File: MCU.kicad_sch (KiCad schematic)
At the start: 34 parts, among them J1 USB_C_Receptacle_USB2.0_16P, SW1 SW_Push, SW2 SW_Push, U1 RP2040, U2 W25Q128JVS, Y1 Crystal_GND24

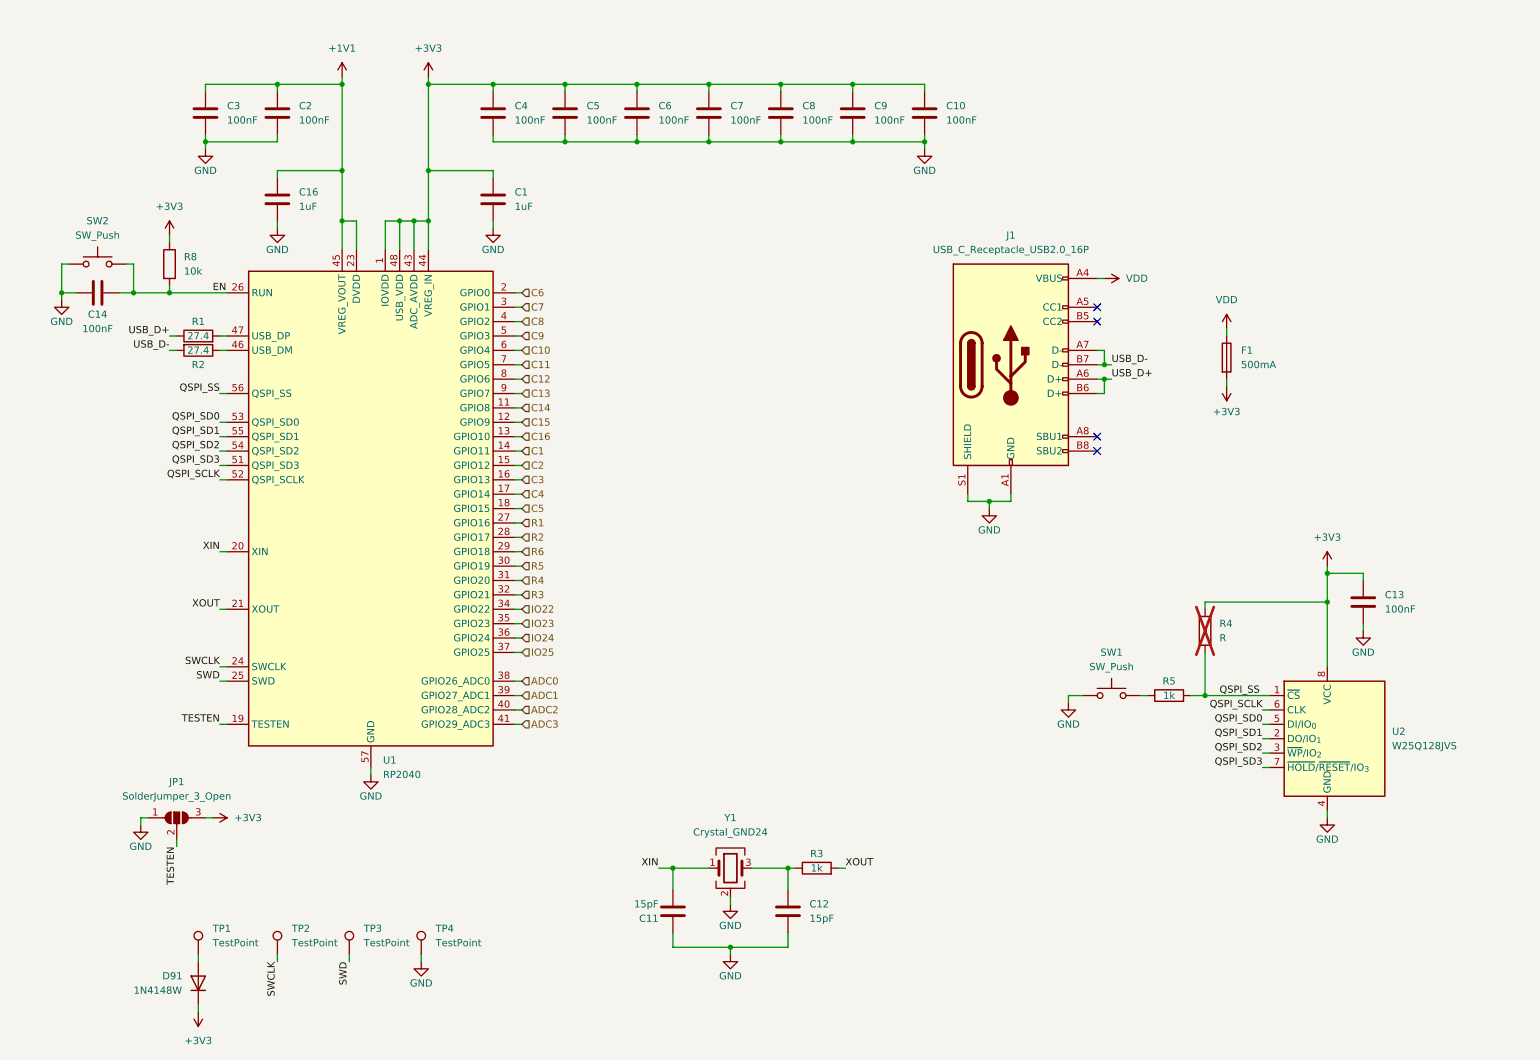
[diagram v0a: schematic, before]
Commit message: Finished V0.1
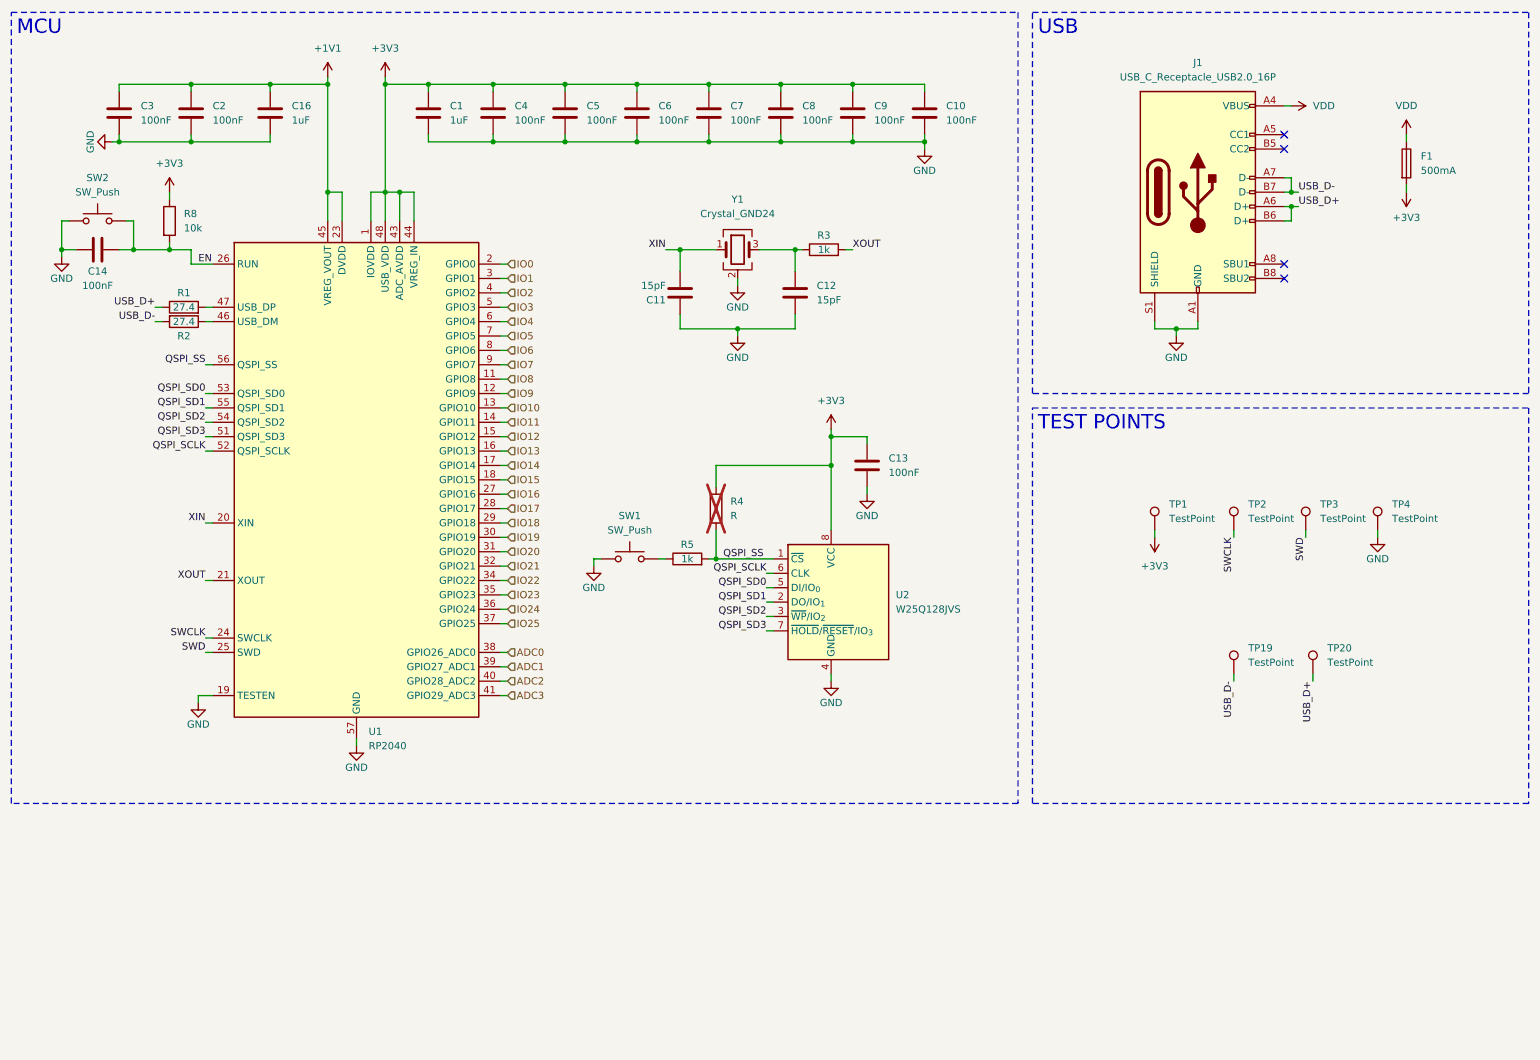
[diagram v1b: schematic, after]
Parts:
- removed D91: 1N4148W, Diode_SMD:D_SOD-123, symbol Diode:1N4148W
- removed JP1: SolderJumper_3_Open, Jumper:SolderJumper-3_P1.3mm_Open_Pad1.0x1.5mm, symbol Jumper:SolderJumper_3_Open
- added TP19, TP20: TestPoint, TestPoint:TestPoint_Pad_D1.0mm, symbol Connector:TestPoint
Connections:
- net TESTEN is gone; now on net GND: U1.19 (TESTEN)
- net +3V3: now also TP1.1
- net USB_D+: now also TP20.1
- net USB_D-: now also TP19.1
- net C1 renamed IO11
- net C10 renamed IO4
- net C11 renamed IO5
- net C12 renamed IO6
- net C13 renamed IO7
- net C14 renamed IO8
- net C15 renamed IO9
- net C16 renamed IO10
- net C2 renamed IO12
- net C3 renamed IO13
- net C4 renamed IO14
- net C5 renamed IO15
- net C6 renamed IO0
- net C7 renamed IO1
- net C8 renamed IO2
- net C9 renamed IO3
- net R1 renamed IO16
- net R2 renamed IO17
- net R3 renamed IO21
- net R4 renamed IO20
- net R5 renamed IO19
- net R6 renamed IO18
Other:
- moved on the sheet: C11, C12, C13, C14, C2, C3, F1, J1, R1, R2, R3, R4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
